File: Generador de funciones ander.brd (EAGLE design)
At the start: 100 x 70 mm, 41 parts, among them IC1 ICL8038, IC2 TL084P, IC3 LF353N

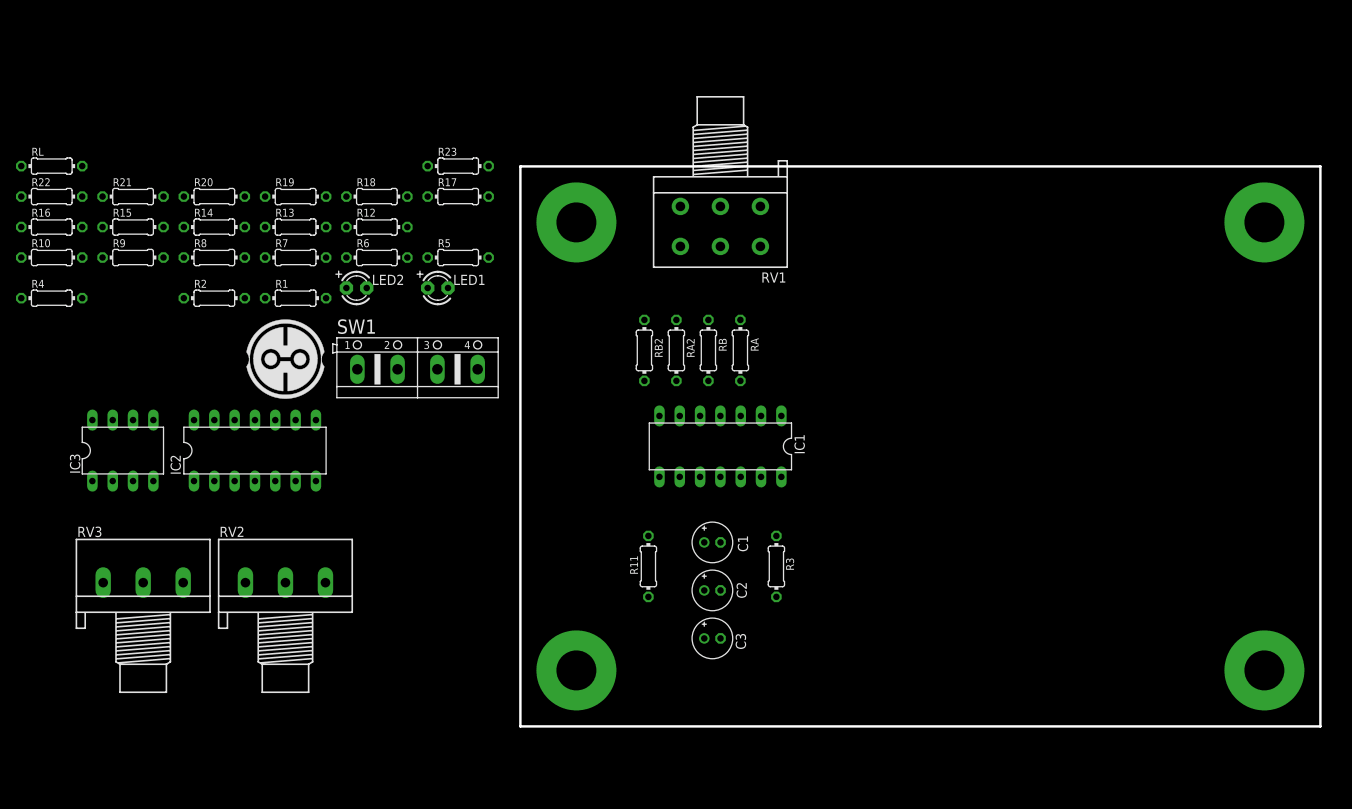
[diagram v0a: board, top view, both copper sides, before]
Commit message: BRD de Andersson con errores. Inicio mi propio BRD
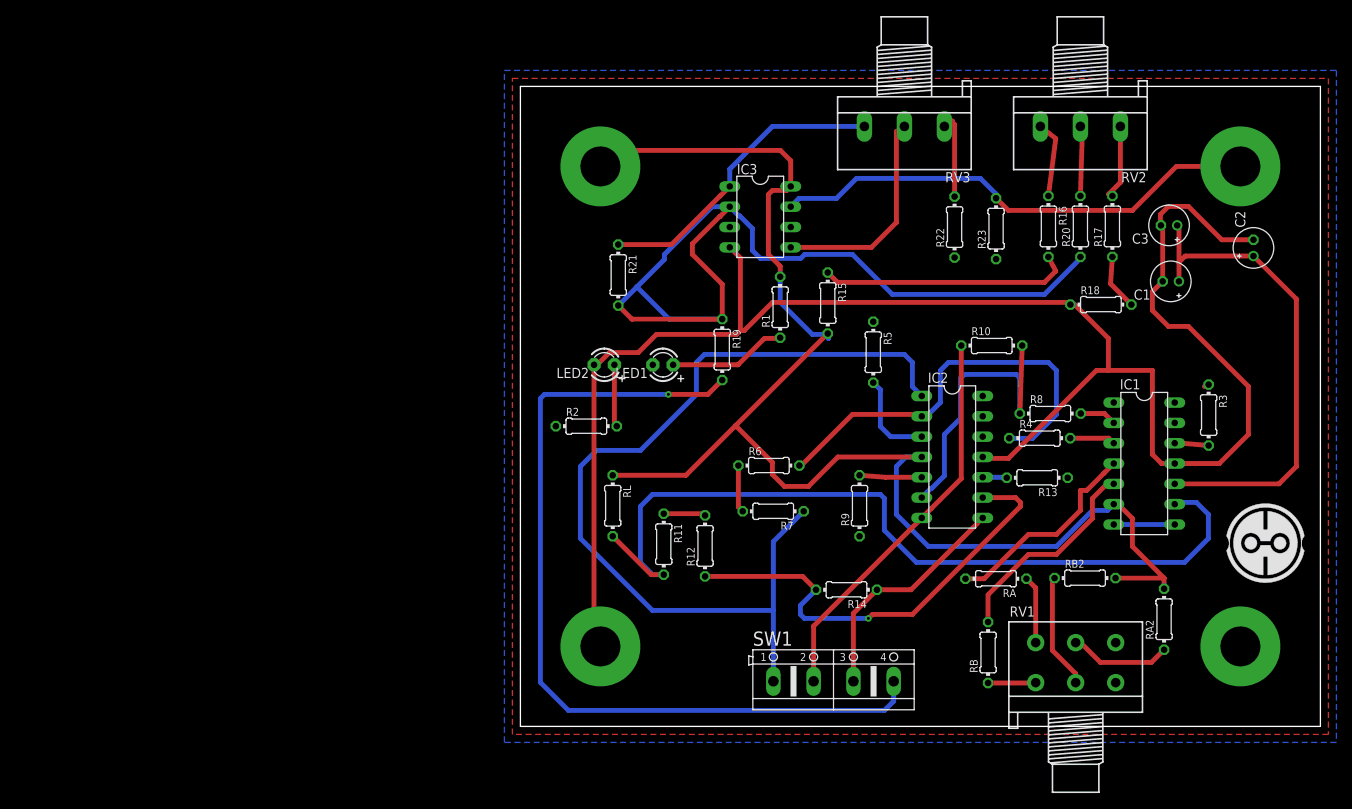
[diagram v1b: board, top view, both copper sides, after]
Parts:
- moved R4 124.7 mm to (64.9, 36.0)
- moved U$1 124.6 mm to (93.1, 22.9)
- moved R16 124.6 mm to (66.0, 62.5), turned to 270 degrees
- moved R10 118.0 mm to (58.9, 47.6)
- moved RV2 114.6 mm to (70.0, 75.0), turned to 180 degrees
- moved R22 112.9 mm to (54.3, 62.4), turned to 90 degrees
- moved RV3 110.9 mm to (48.0, 75.0), turned to 180 degrees
- moved R20 108.3 mm to (70.0, 62.5), turned to 90 degrees
- moved R8 106.3 mm to (66.2, 39.1)
- moved R13 97.9 mm to (64.6, 31.1), turned to 180 degrees
- moved R9 96.0 mm to (42.4, 27.6), turned to 90 degrees
- moved R18 91.5 mm to (72.6, 52.7)
- moved R14 91.1 mm to (40.8, 17.1), turned to 180 degrees
- moved R15 87.4 mm to (38.4, 52.9), turned to 270 degrees
- moved IC2 87.2 mm to (54.0, 33.7), turned to 270 degrees
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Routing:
- net -12V: track 0.00 -> 219.2 mm
- net +12V: track 0.00 -> 177.7 mm
- net N$22: track 0.00 -> 115.9 mm
- net OUT1: track 0.00 -> 114.4 mm
- net N$20: track 0.00 -> 107.7 mm, vias 0 -> 1
- net QUAD: track 0.00 -> 105.6 mm
- net OUT: track 0.00 -> 61.9 mm
- net N$2: track 0.00 -> 61.4 mm
- net N$14: track 0.00 -> 57.4 mm, vias 0 -> 1
- net N$13: track 0.00 -> 53.1 mm
- net OUT2: track 0.00 -> 49.6 mm
- net N$21: track 0.00 -> 38.2 mm
- net N$16: track 0.00 -> 37.7 mm
- net N$23: track 0.00 -> 31.6 mm
- net OUT3: track 0.00 -> 29.6 mm
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- added copper zone on layer 1, net GND
- added copper zone on layer 16, net GND
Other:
- board size 100 x 70 mm -> 100 x 80 mm
